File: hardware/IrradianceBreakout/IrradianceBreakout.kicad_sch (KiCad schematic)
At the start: 2 parts, among them J1 Nano-Fit 1x5

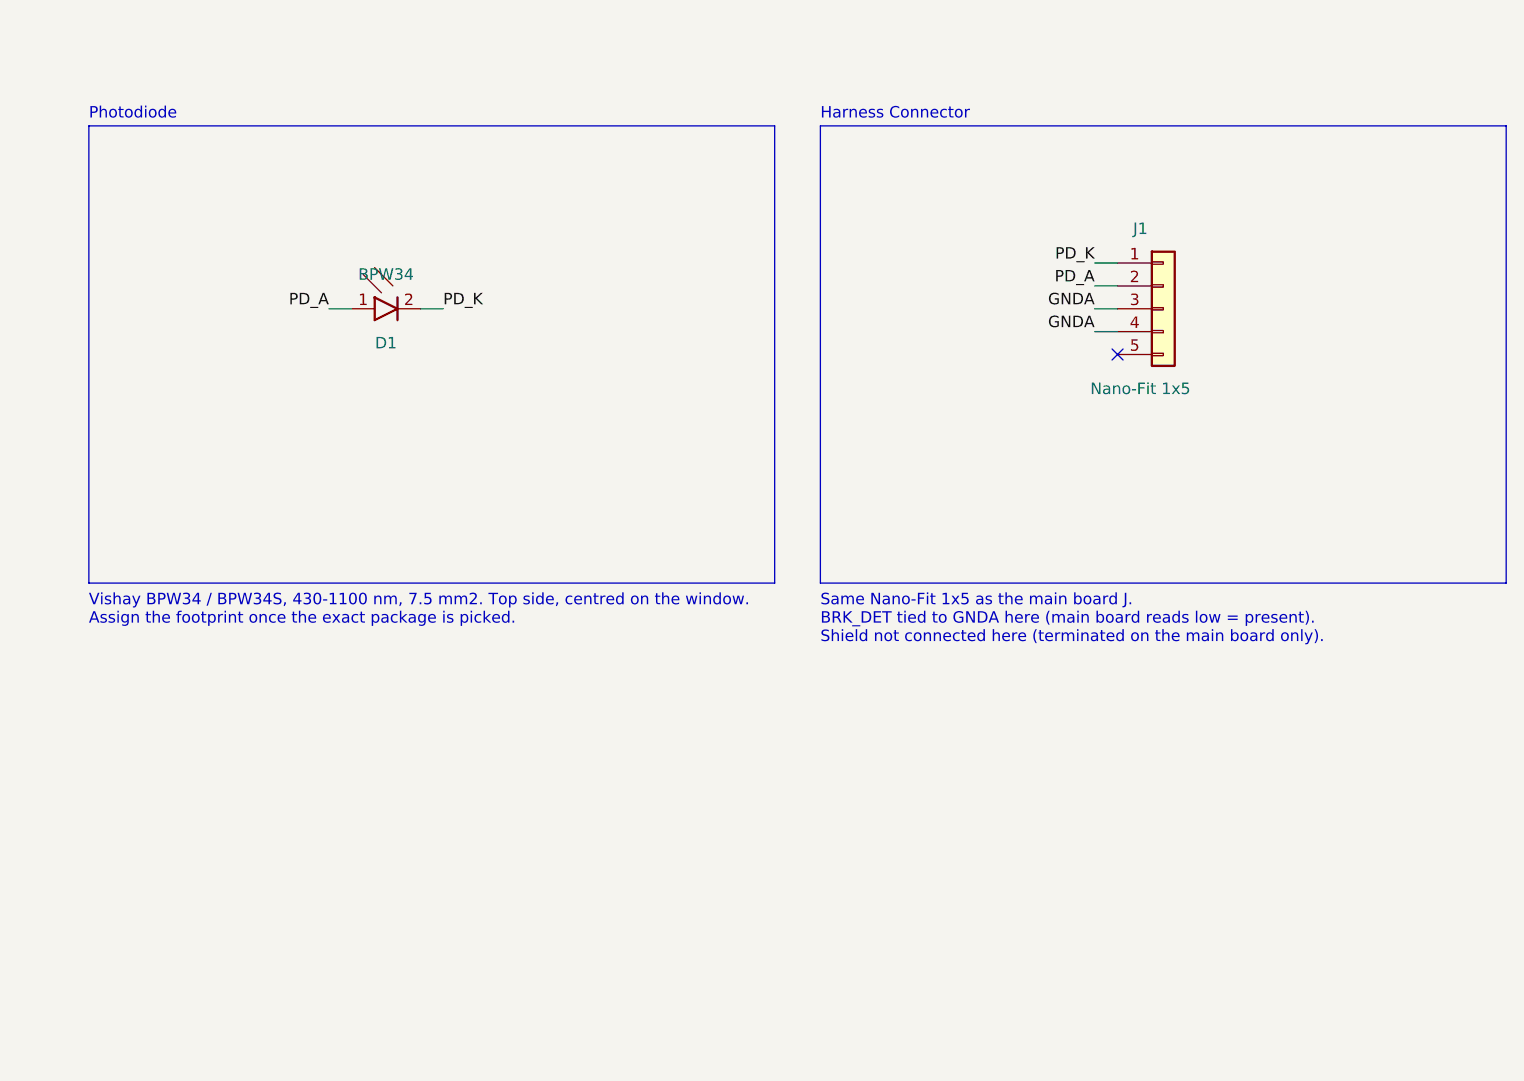
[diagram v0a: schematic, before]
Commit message: updates
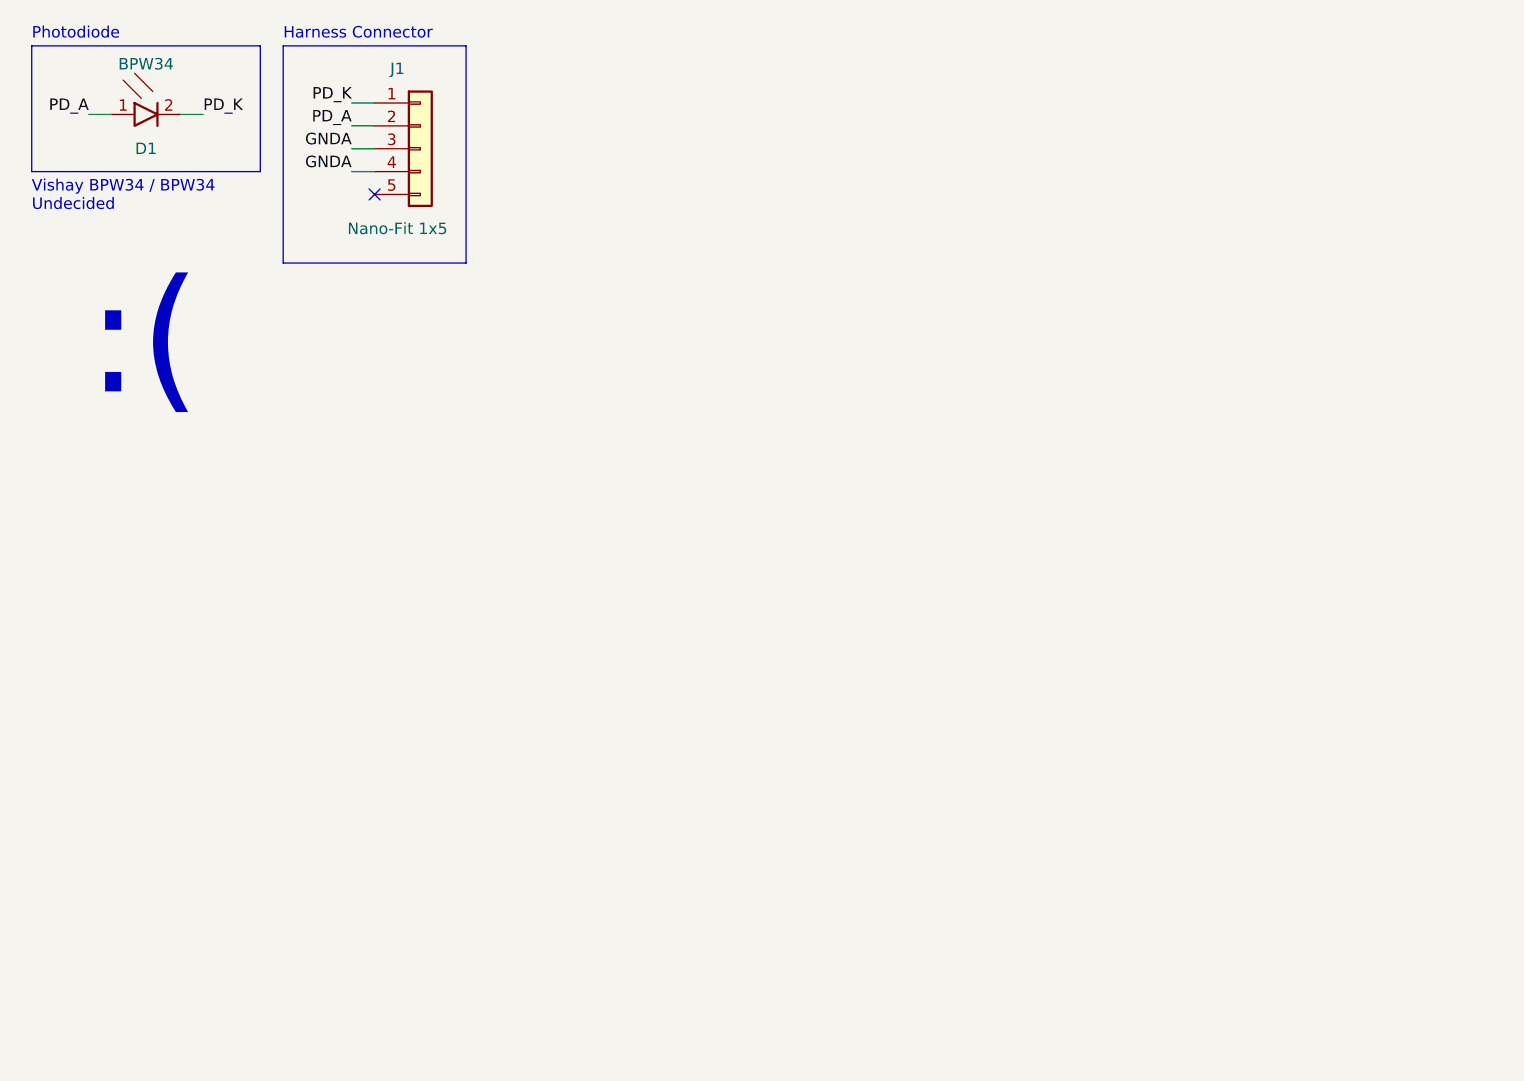
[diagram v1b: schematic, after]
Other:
- note added: ":("
- note added: "Vishay BPW34 / BPW34 Undecided"
- note removed: "Same Nano-Fit 1x5 as the main board J. BRK_DET tied to GNDA here (main board reads low = present). Shield not connected here (terminated on the main board only)."
- note removed: "Vishay BPW34 / BPW34S, 430-1100 nm, 7.5 mm2. Top side, centred on the window. Assign the footprint once the exact package is picked."
- moved on the sheet: D1, J1

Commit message: check breakout board layout
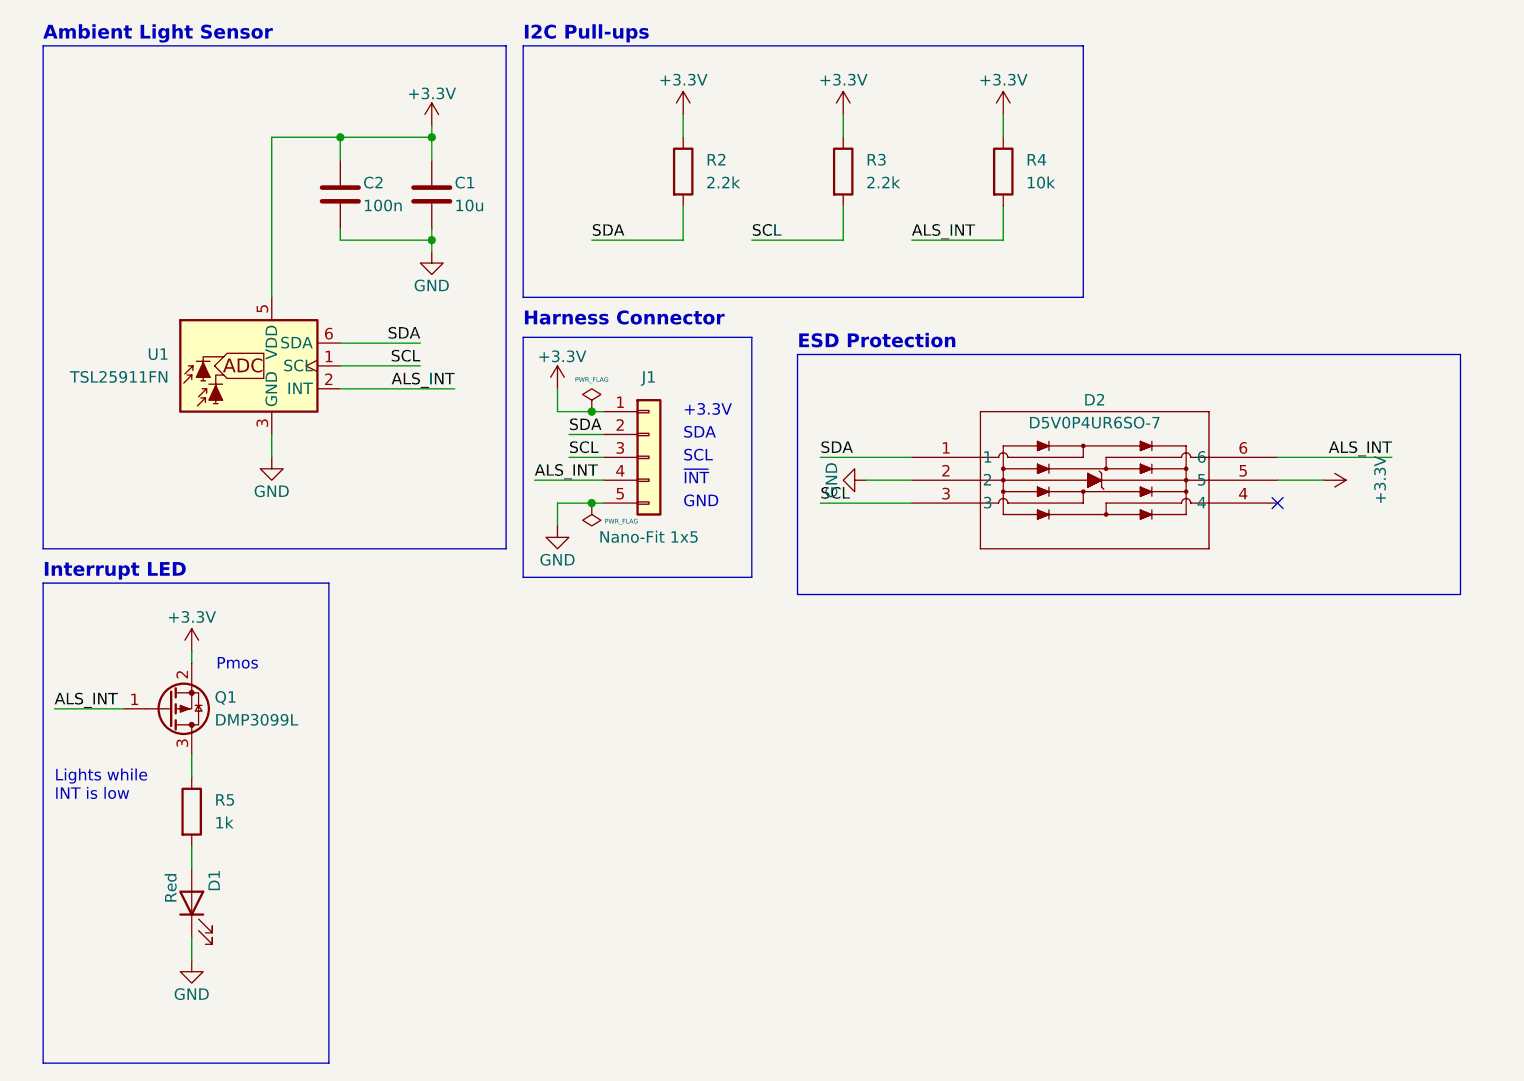
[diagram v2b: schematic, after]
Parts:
- removed D1: BPW34, symbol BlackBody:BPW34
- added C1: 10u, Capacitor_SMD:C_0805_2012Metric_Pad1.18x1.45mm_HandSolder, symbol Device:C
- added C2: 100n, Capacitor_SMD:C_0603_1608Metric_Pad1.08x0.95mm_HandSolder, symbol Device:C
- added D1: Red, LED_SMD:LED_0603_1608Metric, symbol Device:LED
- added D2: D5V0P4UR6SO-7, LHRS_ICs:D5V0P4UR6SO-7, symbol lhrs_ics:D5V0P4UR6SO-7
- added Q1: DMP3099L, Package_TO_SOT_SMD:SOT-23, symbol BlackBody:DMP3099L
- added R2, R3: 2.2k, Resistor_SMD:R_0603_1608Metric_Pad0.98x0.95mm_HandSolder, symbol Device:R
- added R4: 10k, Resistor_SMD:R_0603_1608Metric_Pad0.98x0.95mm_HandSolder, symbol Device:R
- added R5: 1k, Resistor_SMD:R_0603_1608Metric_Pad0.98x0.95mm_HandSolder, symbol Device:R
- added U1: TSL25911FN, OptoDevice:AMS_TSL25911FN, symbol Sensor_Optical:TSL25911FN
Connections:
- net GND: now reaches J1.5 (Pin_5)
- net GND: now also C1.2, C2.2, D1.1 (K), D2.2, U1.3 (GND)
- net GNDA renamed ALS_INT
- net ALS_INT: now also D2.6, Q1.1 (G), R4.2, U1.2 (INT); no longer J1.3 (Pin_3)
- net PD_A renamed SDA
- net SDA: now also D2.1, R2.2, U1.6 (SDA)
- net PD_K renamed +3.3V
- net +3.3V: now also C1.1, C2.1, D2.5, Q1.2 (S), R2.1, R3.1, R4.1, U1.5 (VDD)
- new net: Q1.3 (D), R5.1
- new net: D1.2 (A), R5.2
- new net SCL: D2.3, J1.3 (Pin_3), R3.2, U1.1 (SCL)
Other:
- note added: "+3.3V"
- note added: "Ambient Light Sensor"
- note added: "ESD Protection"
- note added: "GND"
- note added: "I2C Pull-ups"
- note added: "Interrupt LED"
- note added: "Lights while INT is low"
- note added: "Pmos"
- note added: "SCL"
- note added: "SDA"
- note added: "~{INT}"
- note removed: ":("
- note removed: "Photodiode"
- note removed: "Vishay BPW34 / BPW34 Undecided"
